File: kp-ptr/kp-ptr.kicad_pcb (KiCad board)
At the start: 4 copper layers, 31.4 x 101.5 mm, 170 parts, among them IC1 E22-900M22S, J1 ESP32_PROG_CON, J10 Conn_01x02, J11 Conn_01x02, J12 Conn_01x02, J13 Conn_01x02, J2 Conn_01x02, J3 Conn_01x02, J4 USB_C_Receptacle_USB2.0, J5 u.fl, J6 Conn_01x06_Male, J7 Conn_01x10_Male, J8 Conn_01x06_Male, J9 Conn_01x02_Male, Q1 NMOS_SOT23, Q2 DMC2025UFDB_v2, Q3 DMC2025UFDB_v2, Q4 DMC2025UFDB_v2, Q5 DMC2025UFDB_v2, U1 ESP32-S3FN8, U10 USBLC6-2SC6, U11 W25Q128JVS, U12 NL27WZU04DBVT1G, U2 MS560702BA03-50, U3 MMC5983MA, U4 H3LIS331, U5 L76-L, U6 NJG1156PCD, U7 LSM6DSO32, U8 AZ1117CH-5.0TRG1, U9 LDFM33PVR, Y1 7M40000005-40MHz

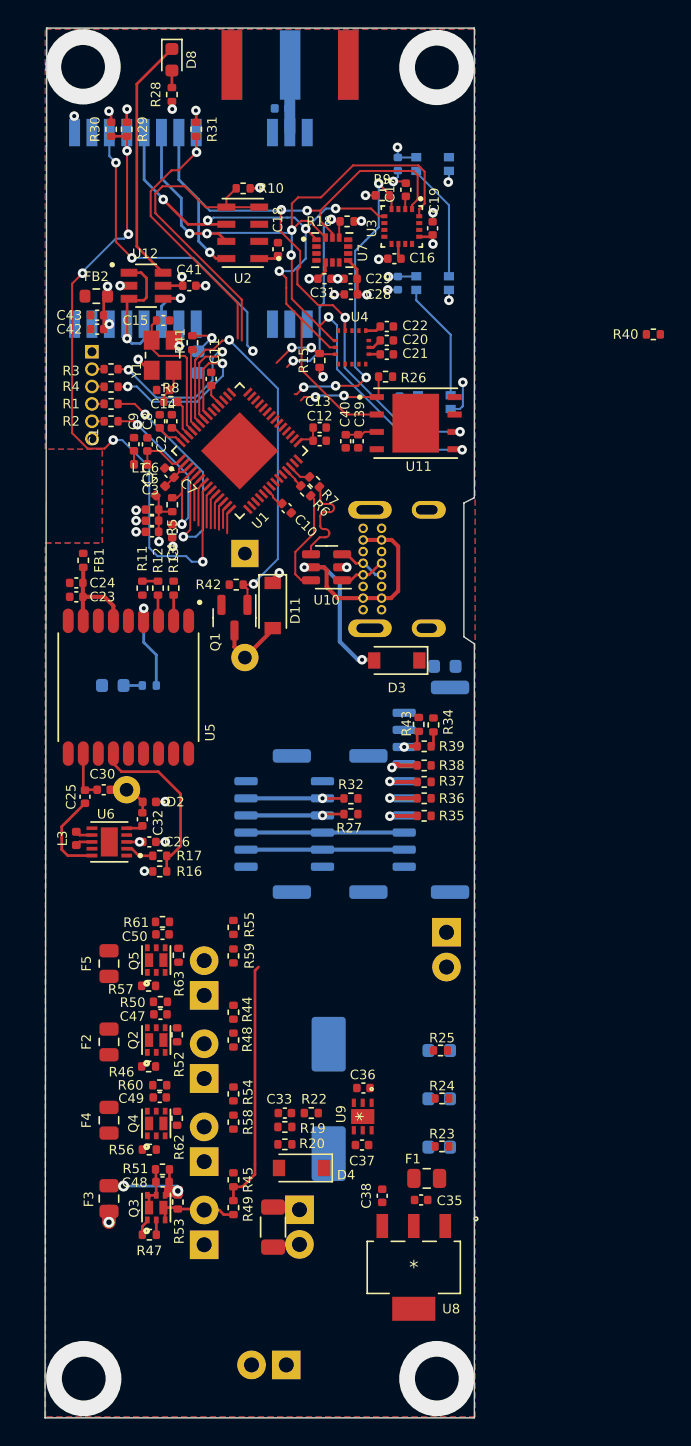
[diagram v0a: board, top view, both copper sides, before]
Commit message: SCH&PCB update
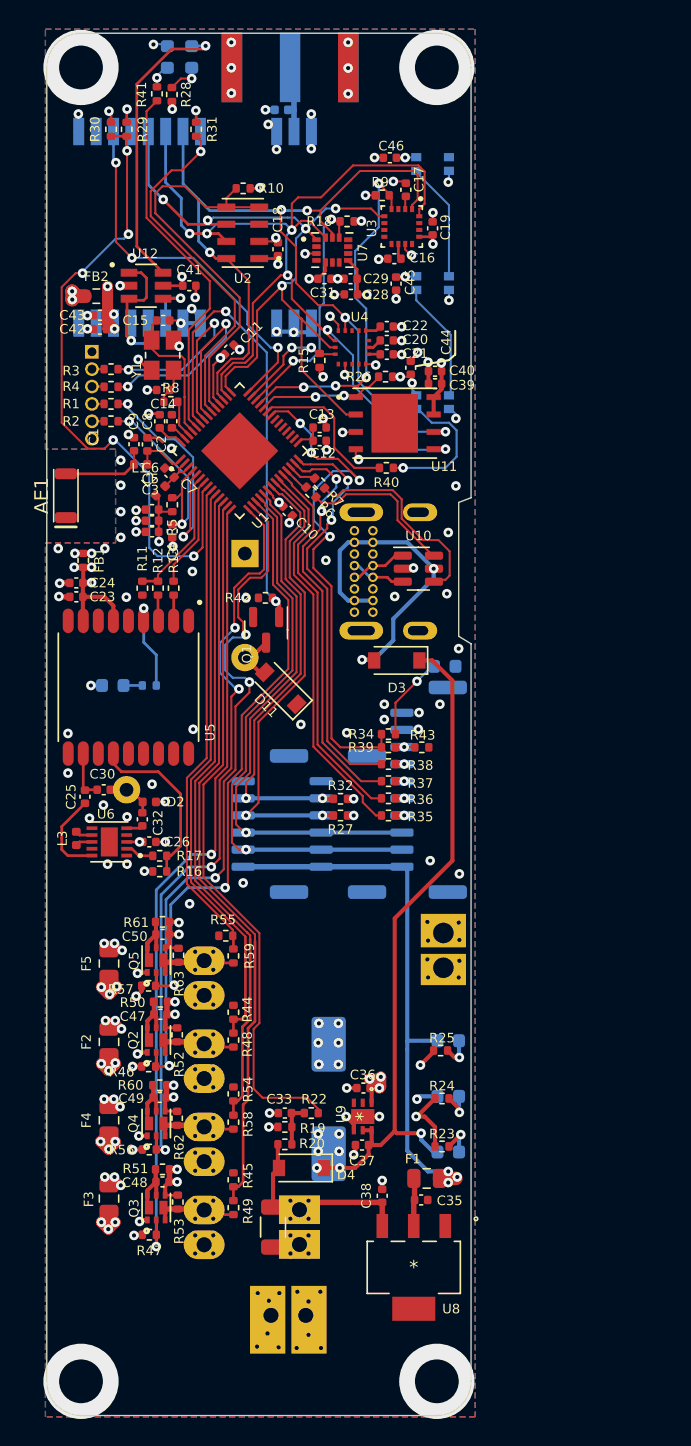
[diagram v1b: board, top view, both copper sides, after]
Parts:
- added AE1: Antenna_Chip, KP-PTR_lib:AMCA31-2R450G-S1F-T3, F.Cu at (142.5, 65.9)
- C44, C45, C46: moved to F.Cu
- D8: moved to B.Cu
- moved D12 22.4 mm to (149.9, 33.8), turned to -90 degrees
- moved R40 21.8 mm to (165.9, 63.9)
- moved R41 18.4 mm to (149.1, 36.5)
- moved C40 8.30 mm to (169.5, 56.8), turned to 180 degrees
- moved C39 7.02 mm to (169.5, 57.7), turned to 180 degrees
- moved U10 6.71 mm to (168.2, 71.2), turned to 0 degrees
- moved D11 6.07 mm to (158.2, 80.0), turned to 135 degrees
- moved J2 3.89 mm to (160.0, 125.8)
- moved R34 3.35 mm to (166.1, 83.3), turned to 180 degrees
- moved C44 2.68 mm to (167.7, 56.5), turned to 90 degrees
- moved R38 2.61 mm to (166.1, 85.5), turned to 180 degrees
- moved R39 2.61 mm to (166.1, 84.3), turned to 180 degrees
- moved R37 2.61 mm to (166.1, 86.7), turned to 180 degrees
- moved R35 2.61 mm to (166.1, 89.3), turned to 180 degrees
- moved R36 2.61 mm to (166.1, 88.0), turned to 180 degrees
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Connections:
- net Net-(C47-Pad1) renamed IGN1_PWR
- net Net-(C48-Pad1) renamed IGN3_PWR
- net Net-(C49-Pad1) renamed IGN2_PWR
- net Net-(C50-Pad1) renamed IGN4_PWR
- J2 pad 1: Earth -> +BATT
- J2 pad 2: +BATT -> Earth
- U1 pad 10: GPIO5 -> IGN1_DET
- U1 pad 11: GPIO6 -> IGN2_DET
- U1 pad 12: GPIO7 -> IGN3_DET
- U1 pad 13: GPIO8 -> VBAT_MEAS
- U1 pad 14: GPIO9 -> IGN3_EN
- U1 pad 15: GPIO10 -> IGN2_EN
- U1 pad 16: GPIO11 -> IGN1_EN
- U1 pad 17: GPIO12 -> IGN4_EN
- U1 pad 18: GPIO13 -> UART1_OUT
- U1 pad 19: GPIO14 -> UART1_IN
- U1 pad 21: GPIO15 -> I2C_SDA
- U1 pad 22: GPIO16 -> I2C_SCL
- U1 pad 23: GPIO17 -> SERVO_1
- U1 pad 24: GPIO18 -> SERVO_2
- U1 pad 27: GPIO21 -> SERVO_3
- U1 pad 28: GPIO26 -> SERVO_4
- U1 pad 36: GPIO48 -> SERVO_EN
- U1 pad 37: GPIO47 -> LED1
- U1 pad 38: GPIO33 -> SPI_CS_FLASH
- U1 pad 39: GPIO34 -> SPI_CS_MAG
- U1 pad 40: GPIO35 -> SPI_CS_LSM
- U1 pad 41: GPIO36 -> SPI_CS_LIS
- U1 pad 42: GPIO37 -> RF_BUSY
- U1 pad 43: GPIO38 -> SPI_MISO
- U1 pad 44: GPIO39 -> SPI_MOSI
- U1 pad 45: GPIO40 -> SPI_CLK
- U1 pad 47: GPIO41 -> SPI_CS_MS5607
- U1 pad 48: GPIO42 -> SPI_CS_LORA
- U1 pad 6: GPIO1 -> GPS_IN
- U1 pad 7: GPIO2 -> GPS_OUT
- U1 pad 9: GPIO4 -> IGN4_DET
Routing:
- net IGN3_EN: track 1.08 -> 58.9 mm, vias 0 -> 2
- net IGN2_EN: track 0.00 -> 55.1 mm, vias 0 -> 4
- net VDD: track 0.00 -> 52.3 mm, vias 0 -> 7
- net IGN1_EN: track 0.00 -> 51.3 mm, vias 0 -> 4
- net VBAT_MEAS: track 0.00 -> 50.9 mm
- net Earth: track 21.7 -> 71.6 mm, vias 23 -> 149
- net IGN2_DET: track 0.00 -> 48.2 mm
- net IGN4_EN: track 0.00 -> 44.0 mm, vias 0 -> 2
- net IGN1_DET: track 0.00 -> 42.5 mm
- net +5V: track 0.00 -> 41.2 mm, vias 0 -> 3
- net SERVO_EN: track 1.12 -> 38.4 mm, vias 0 -> 4
- net IGN3_DET: track 18.2 -> 54.4 mm
- net IGN4_DET: track 0.00 -> 35.8 mm
- net SERVO_4: track 0.00 -> 30.1 mm, vias 0 -> 2
- net SERVO_3: track 0.00 -> 30.0 mm, vias 0 -> 2
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- added copper zone on In2.Cu, net +3.3VADC
- added copper zone on In2.Cu, net +3.3VP
- added copper zone on In2.Cu, net +BATT
- added copper zone on In2.Cu, net IGN1_PWR
- added copper zone on In2.Cu, net IGN2_PWR
- added copper zone on In2.Cu, net IGN3_PWR
- added copper zone on In2.Cu, net IGN4_PWR
- added copper zone on In2.Cu, net VCC
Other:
- board size 31.4 x 101.5 mm -> 31 x 101 mm
- board text added: "+"
- board text added: "3V3"
- board text added: "5V"
- board text added: "ARM"
- board text added: "BAT max 13V"
- board text added: "BOOT"
- board text added: "EN"
- board text added: "GND"
- board text added: "IGN1"
- board text added: "IGN2"
- board text added: "IGN3"
- board text added: "IGN4"
- board text added: "NC"
- board text added: "READY"
- board text added: "RX"
- board text added: "STAT"
- board text added: "SWITCH"
- board text added: "TX"
- board text added: "VIN"
- board text added: "}Vout"
